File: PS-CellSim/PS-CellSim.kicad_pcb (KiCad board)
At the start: 2 copper layers, 49.7 x 59.8 mm, 57 parts, among them J1 bms_taps, J2 bench_vcc, J3 bench_gnd, J4 bms_ref, J5 bms_gpio_set2, J6 bms_gpio_set1, J7 therm_set1, J8 therm_set2

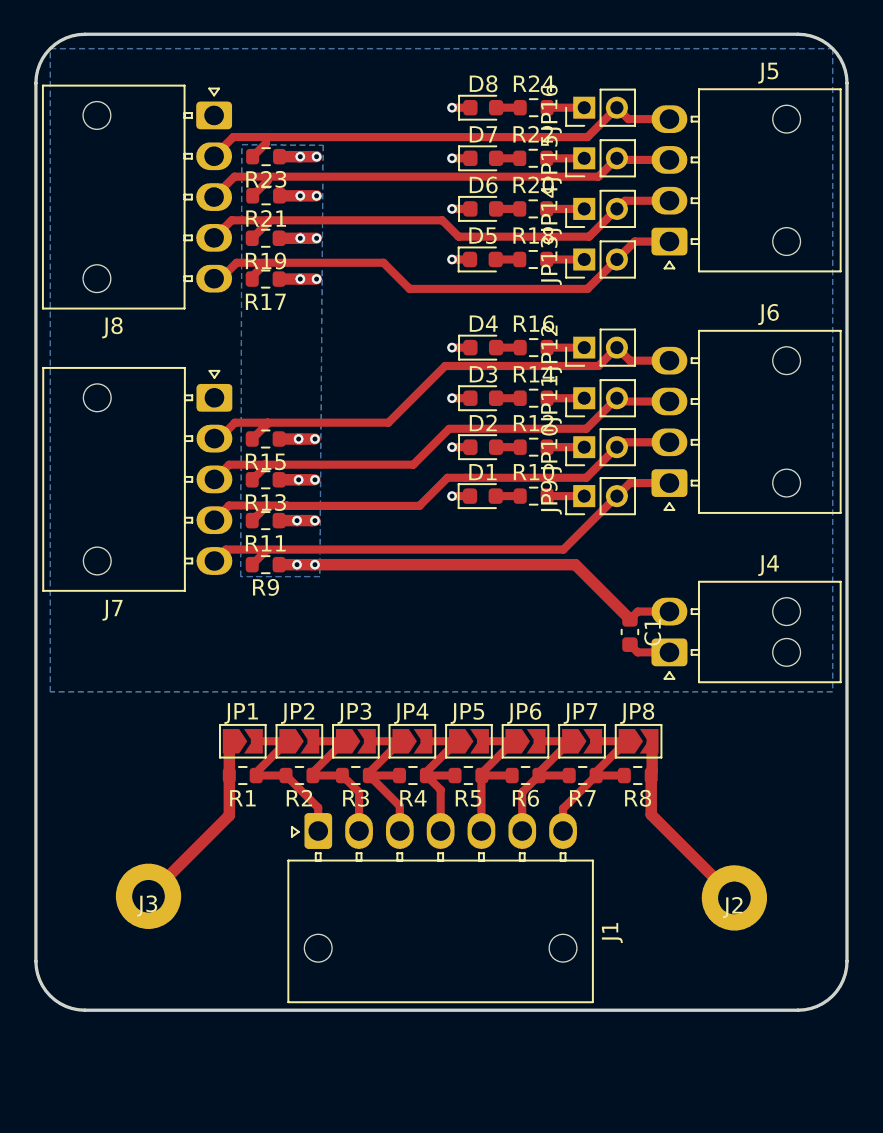
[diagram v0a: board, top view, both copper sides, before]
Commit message: layour layouted
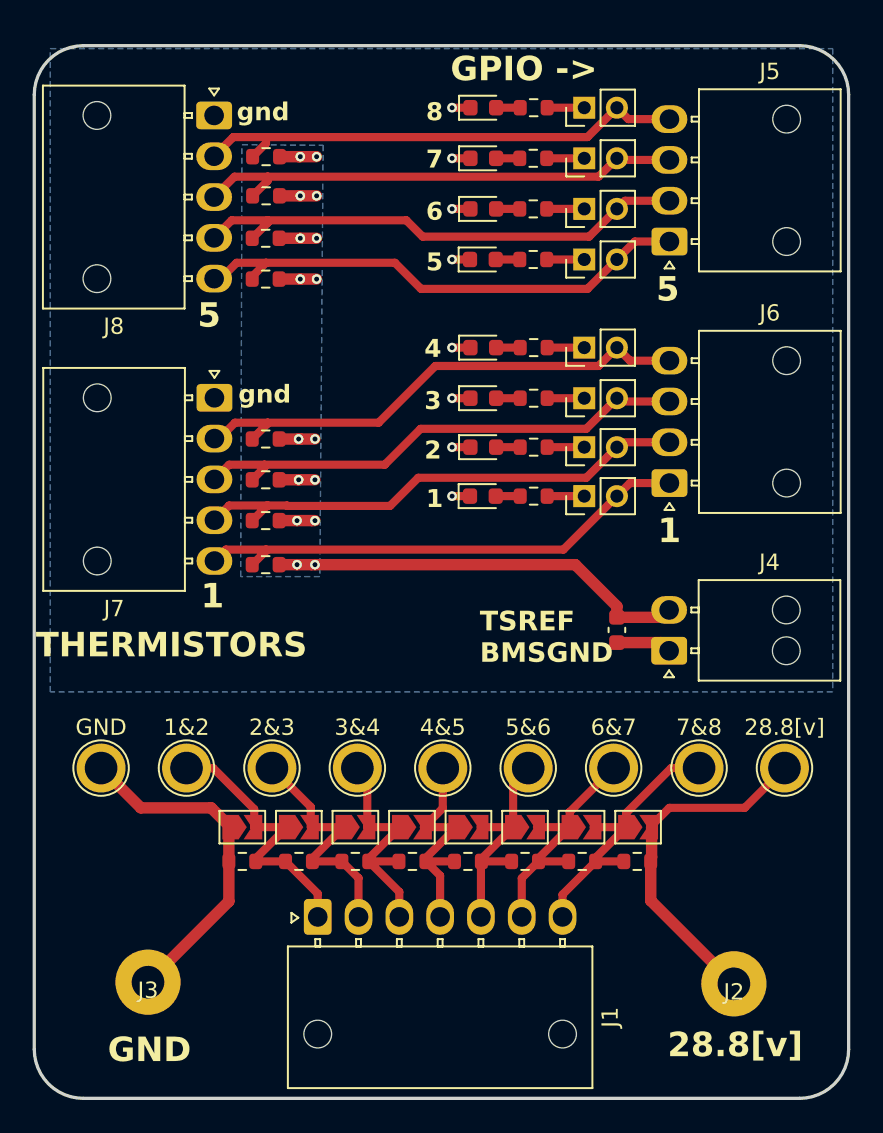
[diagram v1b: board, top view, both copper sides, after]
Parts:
- added 1&2: TestPoint, TestPoint:TestPoint_Plated_Hole_D2.0mm, F.Cu at (128.4, 63.3)
- added 2&3: TestPoint, TestPoint:TestPoint_Plated_Hole_D2.0mm, F.Cu at (133.7, 63.3)
- added 28.8[v]: TestPoint, TestPoint:TestPoint_Plated_Hole_D2.0mm, F.Cu at (165.1, 63.3)
- added 3&4: TestPoint, TestPoint:TestPoint_Plated_Hole_D2.0mm, F.Cu at (138.9, 63.3)
- added 4&5: TestPoint, TestPoint:TestPoint_Plated_Hole_D2.0mm, F.Cu at (144.1, 63.3)
- added 5&6: TestPoint, TestPoint:TestPoint_Plated_Hole_D2.0mm, F.Cu at (149.4, 63.3)
- added 6&7: TestPoint, TestPoint:TestPoint_Plated_Hole_D2.0mm, F.Cu at (154.6, 63.3)
- added 7&8: TestPoint, TestPoint:TestPoint_Plated_Hole_D2.0mm, F.Cu at (159.8, 63.3)
- added GND: TestPoint, TestPoint:TestPoint_Plated_Hole_D2.0mm, F.Cu at (123.2, 63.3)
- moved JP1 5.26 mm to (131.8, 66.9)
- moved JP2 5.26 mm to (135.3, 66.9)
- moved JP3 5.26 mm to (138.8, 66.9)
- moved JP4 5.26 mm to (142.2, 66.9)
- moved JP5 5.26 mm to (145.7, 66.9)
- moved JP6 5.26 mm to (149.2, 66.9)
- moved JP7 5.26 mm to (152.6, 66.9)
- moved JP8 5.26 mm to (156.1, 66.9)
- moved J1 5.26 mm to (151.5, 72.4)
- moved J2 5.26 mm to (162.0, 76.5)
- moved J3 5.26 mm to (126.1, 76.4)
- moved R1 5.26 mm to (131.8, 69.0)
- moved R2 5.26 mm to (135.3, 69.0)
- moved R3 5.26 mm to (138.8, 69.0)
- moved R4 5.26 mm to (142.3, 69.0)
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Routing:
- net VCC: track 11.7 -> 21.5 mm
- net GND: track 11.6 -> 21.0 mm
- net /7&8: track 10.9 -> 17.3 mm
- net /1&2: track 11.1 -> 17.4 mm
- net /6&7: track 10.8 -> 15.5 mm
- net /2&3: track 10.5 -> 15.1 mm
- net /4&5: track 10.4 -> 14.5 mm
- net /5&6: track 10.2 -> 14.2 mm
- net /3&4: track 10.9 -> 14.8 mm
- net GND1: track 11.6 -> 12.4 mm
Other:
- board size 49.7 x 59.8 mm -> 49.9 x 64.5 mm
- board text added: "1"
- board text added: "2"
- board text added: "28.8[v]"
- board text added: "3"
- board text added: "4"
- board text added: "5"
- board text added: "6"
- board text added: "7"
- board text added: "8"
- board text added: "GND"
- board text added: "GPIO ->"
- board text added: "THERMISTORS"
- board text added: "TSREF BMSGND"
- board text added: "gnd"
